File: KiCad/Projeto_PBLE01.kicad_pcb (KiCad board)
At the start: 2 copper layers, 84 parts, among them IC1 LM358

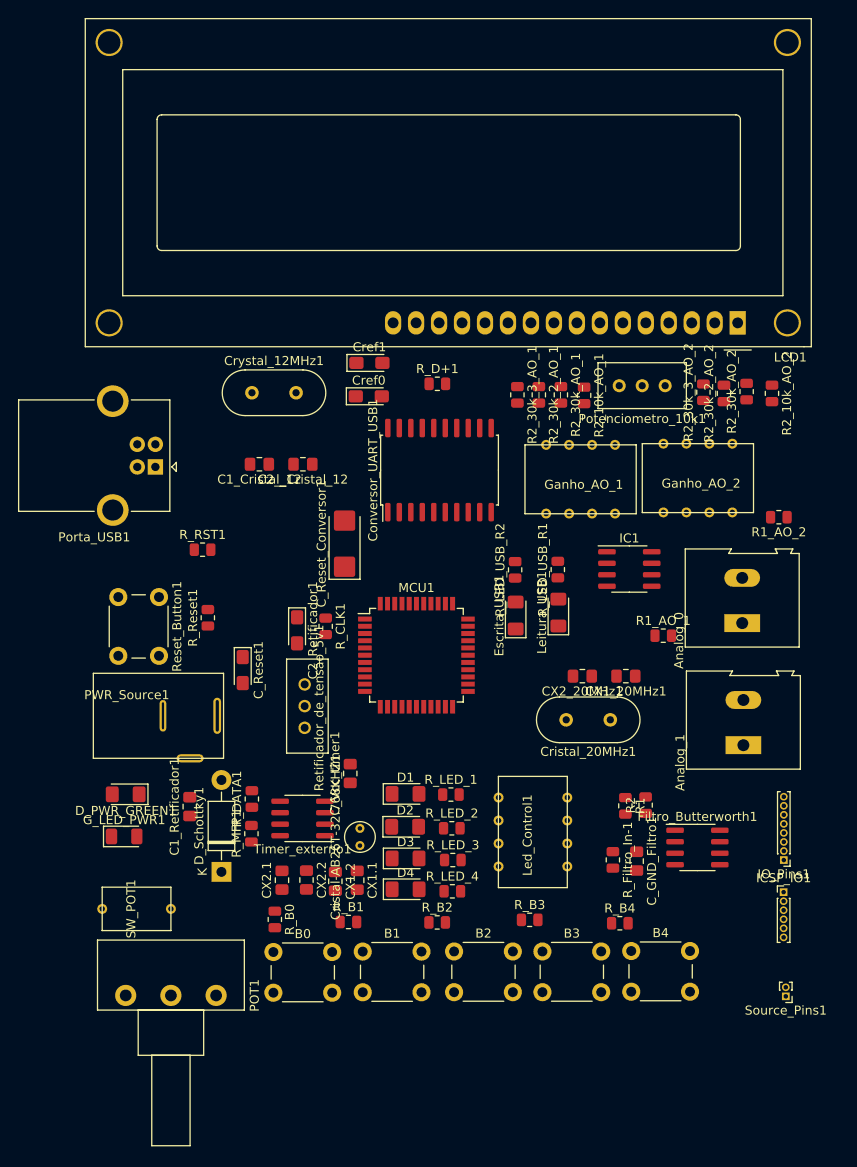
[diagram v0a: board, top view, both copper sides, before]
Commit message: Trilhas
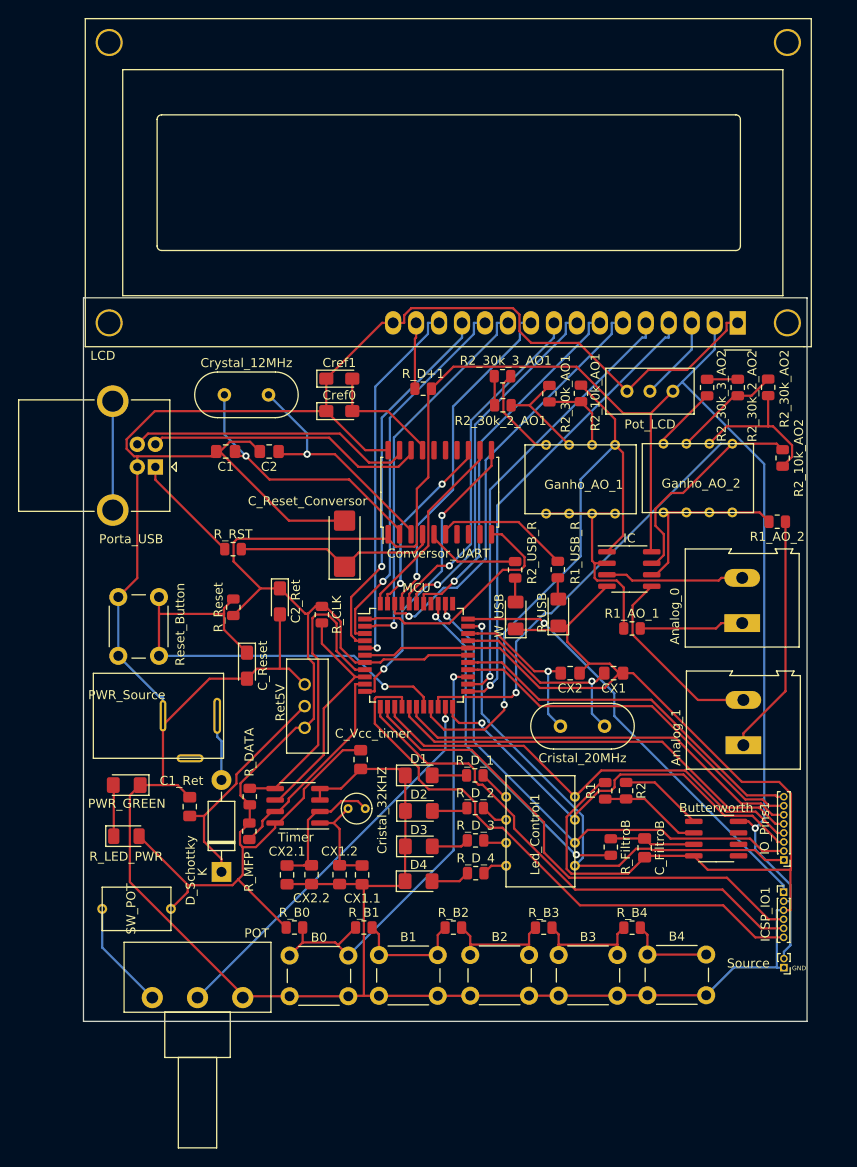
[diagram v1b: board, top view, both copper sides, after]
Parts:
- moved R2_10k_AO2 7.24 mm to (129.4, 93.9), turned to 90 degrees
- moved Cristal_32KHZ 4.29 mm to (81.3, 132.7), turned to 0 degrees
- moved R2_30k_2_AO1 4.14 mm to (98.4, 88.1), turned to 180 degrees
- moved C1 3.99 mm to (67.8, 93.2)
- moved C2 3.99 mm to (72.6, 93.2)
- moved Cref1 3.76 mm to (80.4, 85.1)
- moved C2_Ret 3.72 mm to (73.8, 109.8)
- moved Cref0 3.65 mm to (80.4, 88.7)
- moved R1_AO_1 3.55 mm to (112.7, 112.8)
- moved R_D_2 3.42 mm to (95.4, 132.6)
- moved R_D_1 3.39 mm to (95.3, 129.0)
- moved R_RST 3.37 mm to (68.6, 104.0)
- moved R_D_3 3.32 mm to (95.4, 136.2)
- moved R_D_4 3.27 mm to (95.4, 139.8)
- moved Source 3.18 mm to (129.5, 150.3)
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- renumbered Filtro_Butterworth1 to Butterworth, C1_Cristal_12 to C1, C1_Retificador1 to C1_Ret, C2__Cristal_12 to C2, C2_Retificador1 to C2_Ret, CX1_20MHz1 to CX1, CX2_20MHz1 to CX2, C_GND_Filtro1 to C_FiltroB, C_Reset1 to C_Reset, C_Reset_Conversor1 to C_Reset_Conversor, C_Vcc_timer1 to C_Vcc_timer, Conversor_UART_USB1 to Conversor_UART, Cristal_20MHz1 to Cristal_20MHz, Cristal-AB26T-32.768KHZ1 to Cristal_32KHZ, Crystal_12MHz1 to Crystal_12MHz, D_Schottky1 to D_Schottky, IC1 to IC, LCD1 to LCD, MCU1 to MCU, POT1 to POT, D_PWR_GREEN1 to PWR_GREEN, PWR_Source1 to PWR_Source, Porta_USB1 to Porta_USB, Potenciometro_10k1 to Pot_LCD, R_LED_USB_R1 to R1_USB_R, R2_10k_AO_1 to R2_10k_AO1, R2_10k_AO_2 to R2_10k_AO2, R2_30k_2_AO_1 to R2_30k_2_AO1, R2_30k_2_AO_2 to R2_30k_2_AO2, R2_30k_3_AO_1 to R2_30k_3_AO1, R2_30k_3_AO_2 to R2_30k_3_AO2, R2_30k_AO_1 to R2_30k_AO1, R2_30k_AO_2 to R2_30k_AO2, R_LED_USB_R2 to R2_USB_R, R_CLK1 to R_CLK, R_DATA1 to R_DATA, R_LED_1 to R_D_1, R_LED_2 to R_D_2, R_LED_3 to R_D_3, R_LED_4 to R_D_4, R_Filtro_In-1 to R_FiltroB, G_LED_PWR1 to R_LED_PWR, R_MFP1 to R_MFP, R_RST1 to R_RST, R_Reset1 to R_Reset, Leitura_USB1 to R_USB, Reset_Button1 to Reset_Button, Retificador_de_tensão_5v1 to Ret5V, SW_POT1 to SW_POT, Source_Pins1 to Source, Timer_externo1 to Timer, Escrita_USB1 to W_USB
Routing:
- net GNDREF: track 0.00 -> 474.3 mm
- net Vcc_5v: track 0.00 -> 284.8 mm, vias 0 -> 1
- net /Analog_1: track 0.00 -> 73.0 mm, vias 0 -> 1
- net /Analog_0: track 0.00 -> 66.2 mm, vias 0 -> 1
- net /ICSP_Enable: track 0.00 -> 63.4 mm
- net /IO_00: track 0.00 -> 57.4 mm, vias 0 -> 1
- net /IO_01: track 0.00 -> 57.0 mm, vias 0 -> 1
- net /ICSP_Clk: track 0.00 -> 56.9 mm
- net /ICSP_Data: track 0.00 -> 56.1 mm
- net /MCLR: track 0.00 -> 53.3 mm, vias 0 -> 1
- net /IO_03: track 0.00 -> 51.8 mm
- net /LCD_RS: track 0.00 -> 51.2 mm, vias 0 -> 1
- net /Analog_KB: track 0.00 -> 49.3 mm, vias 0 -> 1
- net /ICSP_RST: track 0.00 -> 49.3 mm, vias 0 -> 1
- net /LCD_RW: track 0.00 -> 49.2 mm, vias 0 -> 1
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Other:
- board outline added: 80 x 80 mm
- rule via_min_size: 0.4 -> 0.6
- board text added: "GND"
